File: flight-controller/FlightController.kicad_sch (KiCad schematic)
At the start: 30 parts, among them J1 USB_C_Receptacle_USB2.0_14P, J2 Conn_01x03_Pin, J3 Conn_01x03_Pin, J4 Conn_01x03_Pin, J5 Conn_01x03_Pin, J7 Micro_SD_Card_Det1, J8 Conn_01x06_Pin, U1 ESP32-S3-WROOM-1, U2 TPS629210DRLR, U3 MMC5983MA, U4 BMI270, U5 BMP581

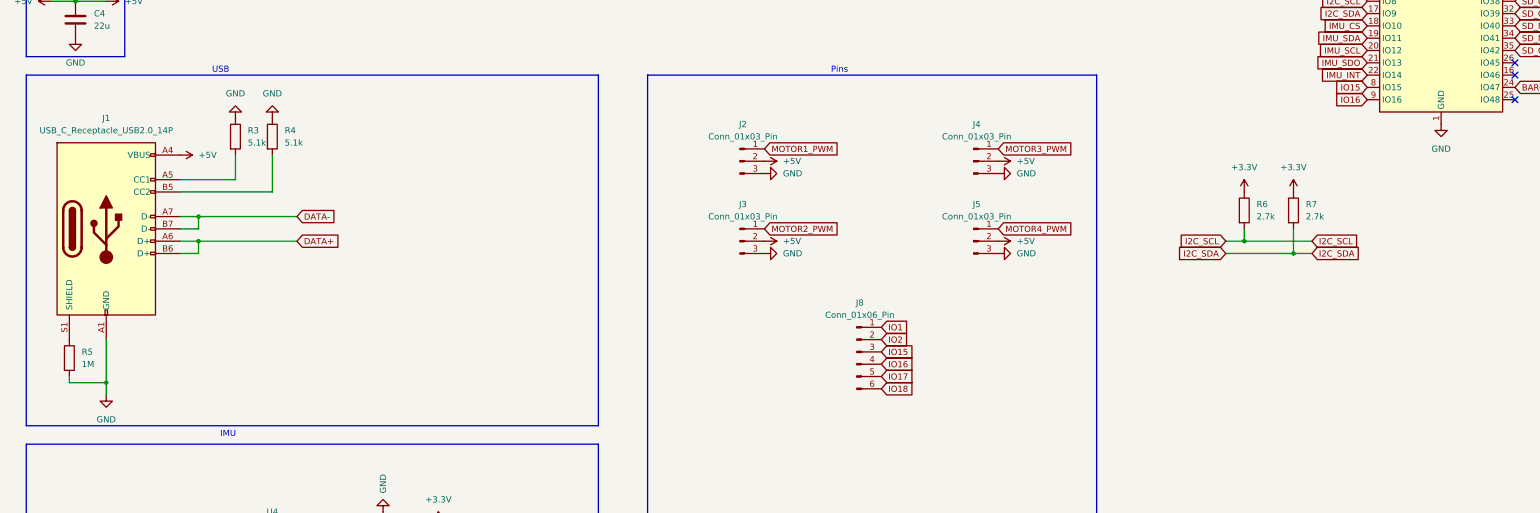
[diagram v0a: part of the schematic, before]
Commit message: update usb
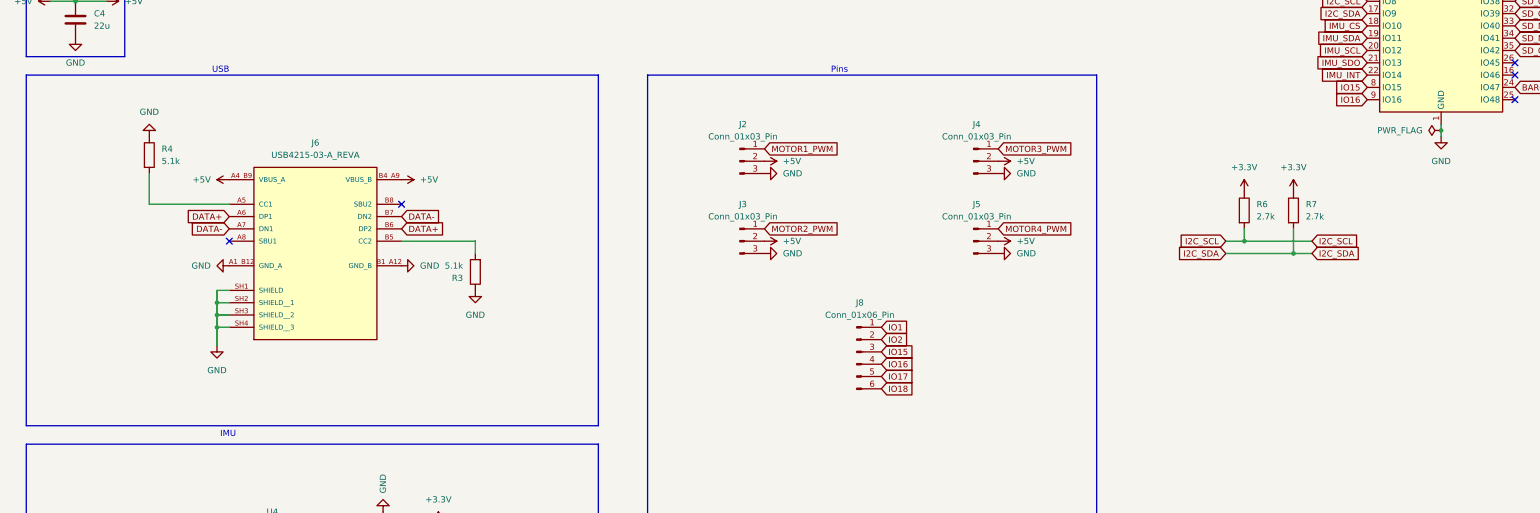
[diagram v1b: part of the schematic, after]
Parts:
- removed J1: USB_C_Receptacle_USB2.0_14P, symbol Connector:USB_C_Receptacle_USB2.0_14P
- removed R5: 1M, symbol Device:R
- added J6: USB4215-03-A_REVA, USB4215-03-A_REVA:GCT_USB4215-03-A_REVA, symbol USB4215-03-A_REVA:USB4215-03-A_REVA
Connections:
- net +5V: now also J6.A4_B9 (VBUS_A), J6.B4_A9 (VBUS_B)
- net DATA+: now also J6.A6 (DP1), J6.B6 (DP2)
- net DATA-: now also J6.A7 (DN1), J6.B7 (DN2)
- net GND: now also J6.A1_B12 (GND_A), J6.B1_A12 (GND_B), J6.SH1 (SHIELD), J6.SH2 (SHIELD__1), J6.SH3 (SHIELD__2), J6.SH4 (SHIELD__3)
- net at R3.2: now also J6.B5 (CC2)
- net at R4.2: now also J6.A5 (CC1)
- no-connect marks 21 -> 23
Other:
- moved on the sheet: R4

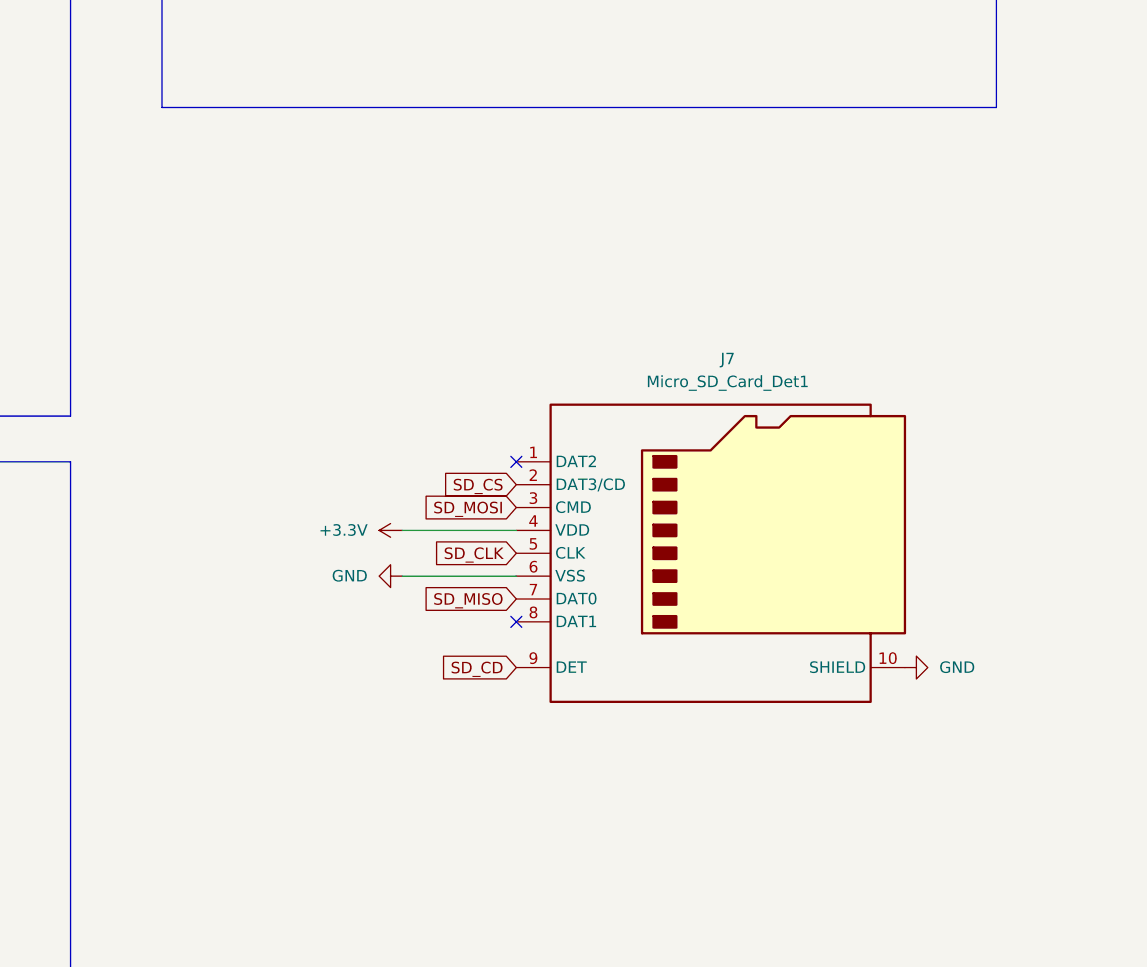
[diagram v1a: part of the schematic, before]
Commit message: add footprints
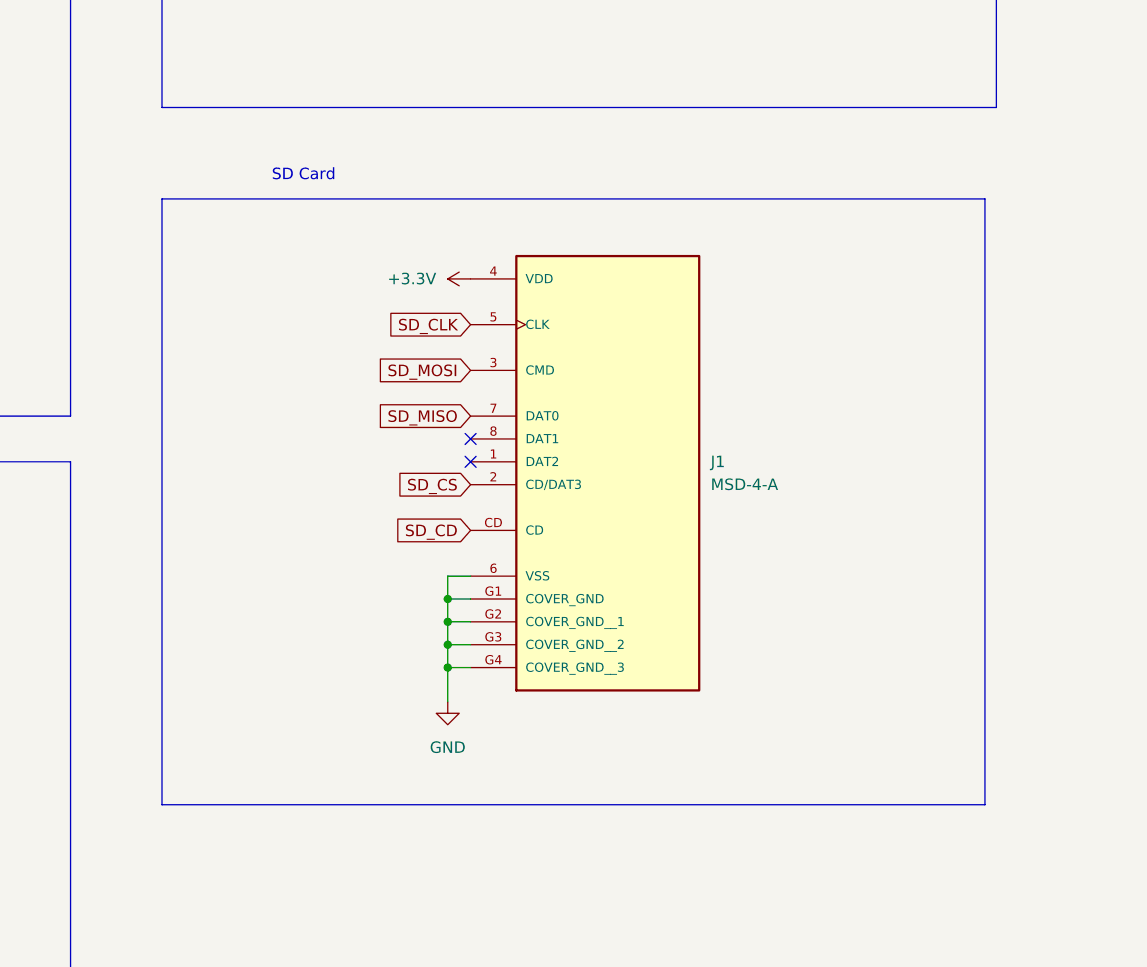
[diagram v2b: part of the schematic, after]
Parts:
- removed J7: Micro_SD_Card_Det1, symbol Connector:Micro_SD_Card_Det1
- added J1: MSD-4-A, MSD-4-A:CUI_MSD-4-A, symbol MSD-4-A:MSD-4-A
- C1, C10, C2, C3, C4, C5, C6, C7, C8, C9: footprint (none) -> Capacitor_SMD:C_0603_1608Metric_Pad1.08x0.95mm_HandSolder
- J2, J3, J4, J5: footprint (none) -> Connector_PinHeader_2.54mm:PinHeader_1x03_P2.54mm_Vertical
- J8: footprint (none) -> Connector_PinHeader_2.54mm:PinHeader_1x06_P2.54mm_Vertical
- L1: footprint (none) -> Inductor_SMD:L_1008_2520Metric_Pad1.43x2.20mm_HandSolder
- R1, R2, R3, R4, R6, R7: footprint (none) -> Resistor_SMD:R_0603_1608Metric_Pad0.98x0.95mm_HandSolder
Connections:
- net +3.3V: now also J1.4 (VDD)
- net GND: now also J1.6 (VSS), J1.G1 (COVER_GND), J1.G2 (COVER_GND__1), J1.G3 (COVER_GND__2), J1.G4 (COVER_GND__3)
- net SD_CD: now also J1.CD
- net SD_CLK: now also J1.5 (CLK)
- net SD_CS: now also J1.2 (CD/DAT3)
- net SD_MISO: now also J1.7 (DAT0)
- net SD_MOSI: now also J1.3 (CMD)
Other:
- note added: "SD Card"

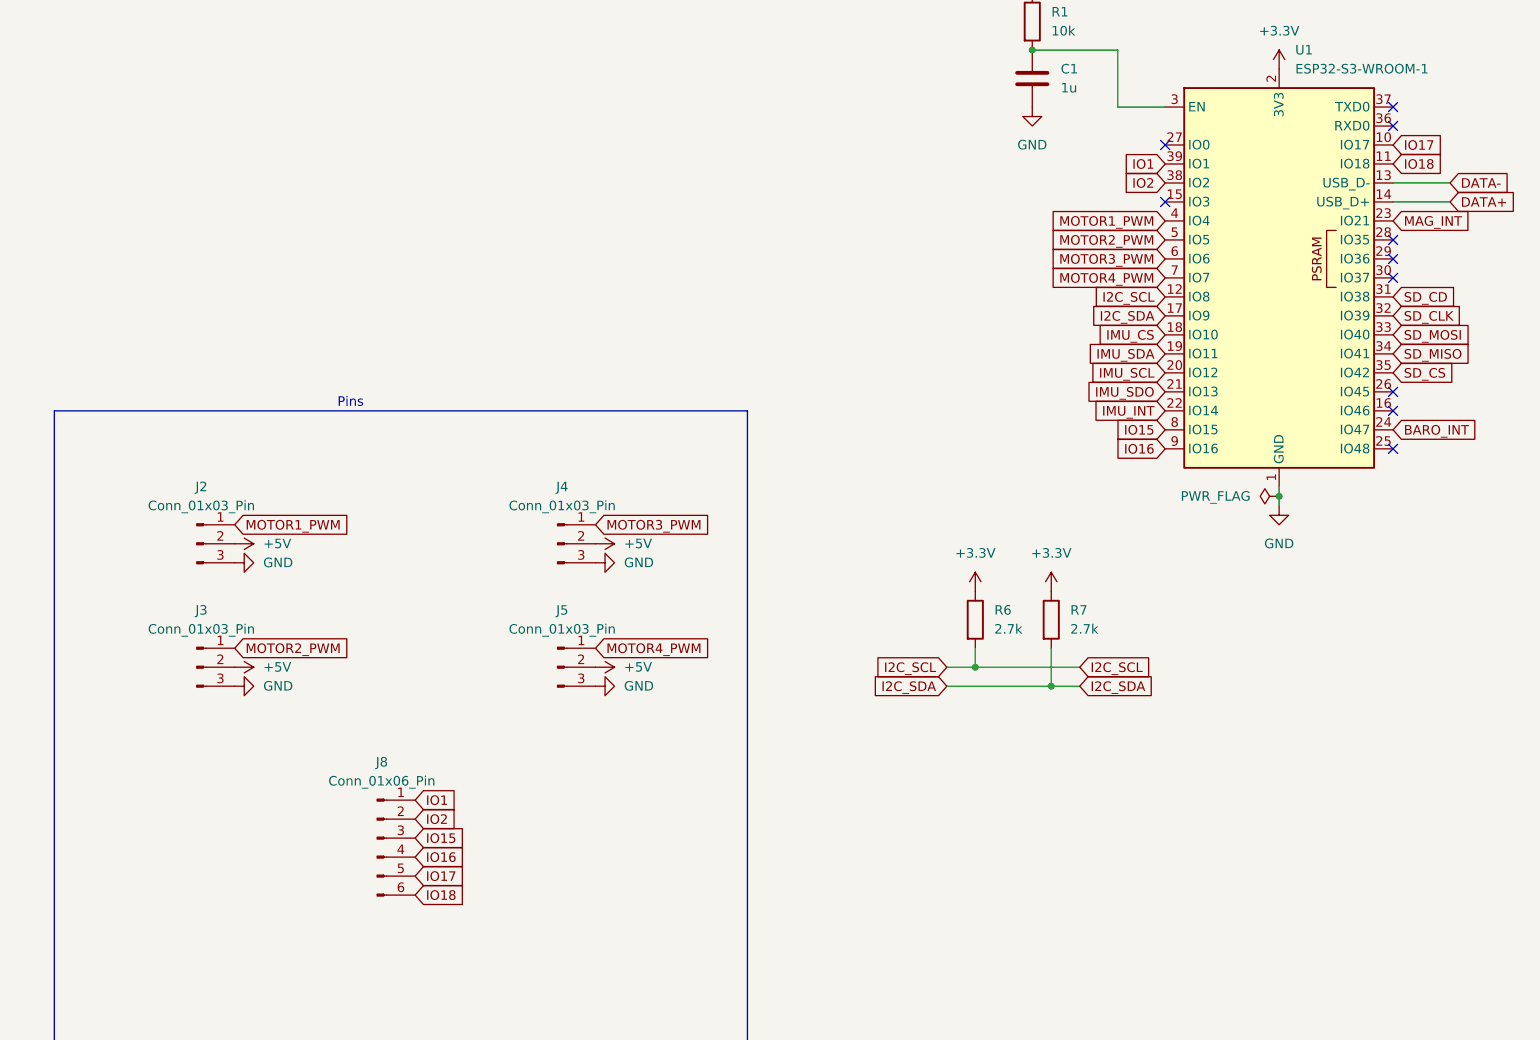
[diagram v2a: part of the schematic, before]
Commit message: general component locations
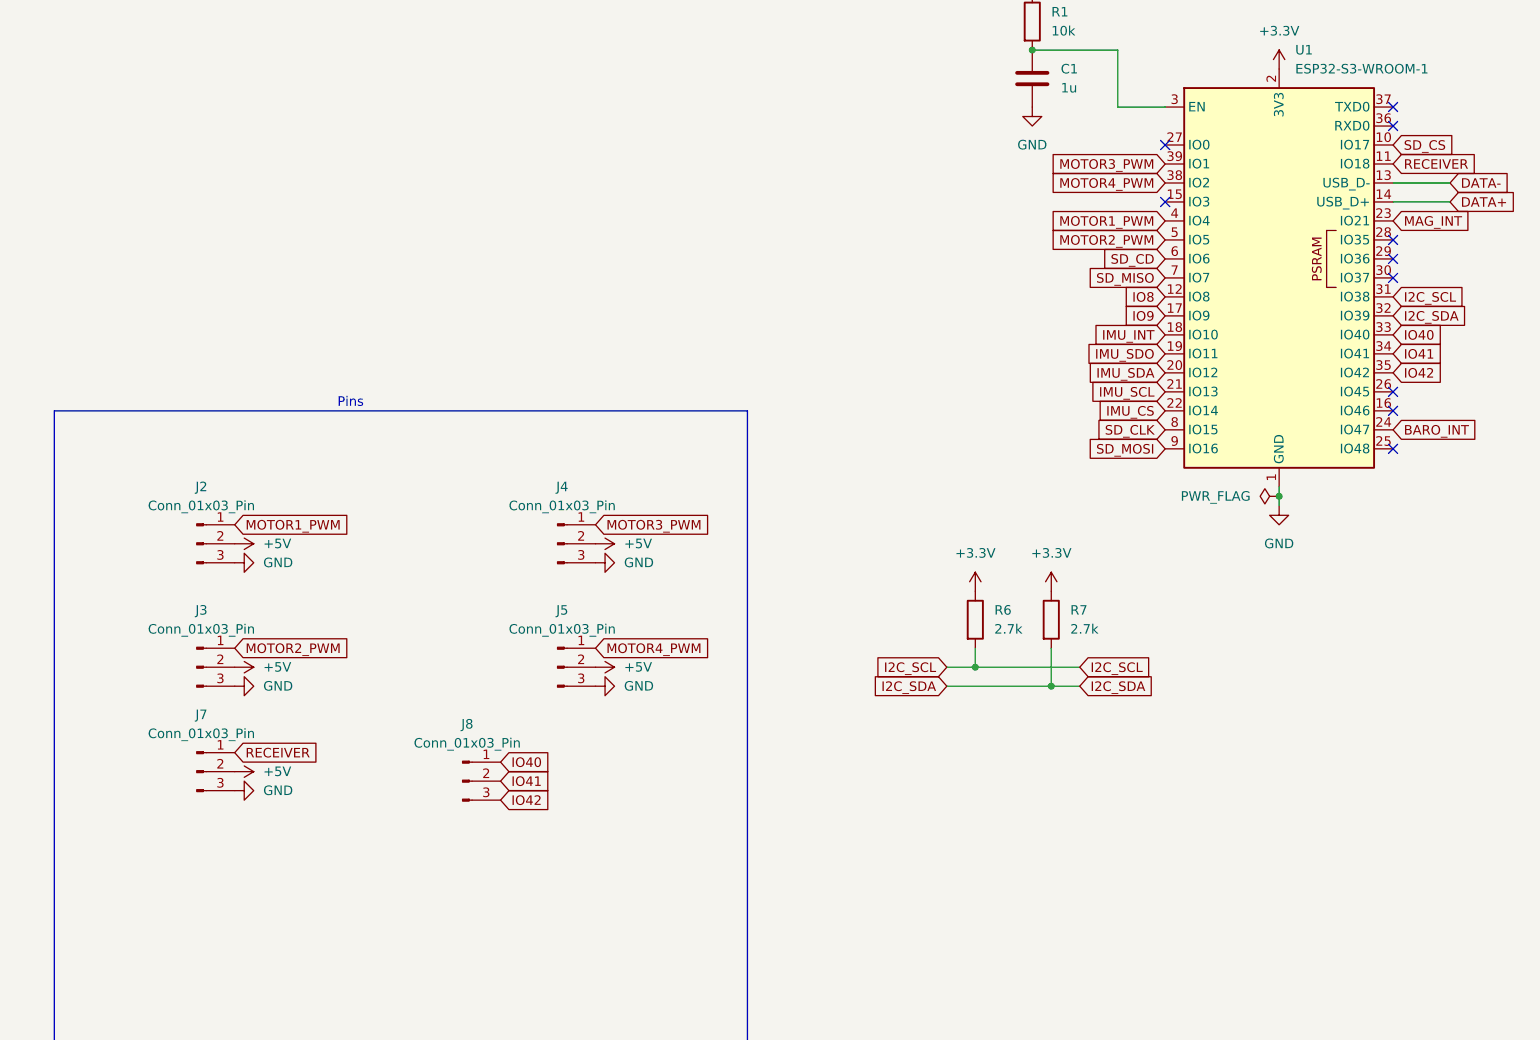
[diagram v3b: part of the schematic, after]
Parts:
- removed J8: Conn_01x06_Pin, Connector_PinHeader_2.54mm:PinHeader_1x06_P2.54mm_Vertical, symbol Connector:Conn_01x06_Pin
- added J7, J8: Conn_01x03_Pin, Connector_PinHeader_2.54mm:PinHeader_1x03_P2.54mm_Vertical, symbol Connector:Conn_01x03_Pin
- J1: footprint MSD-4-A:CUI_MSD-4-A -> MSD_4_A:CUI_MSD-4-A
- J6: footprint USB4215-03-A_REVA:GCT_USB4215-03-A_REVA -> USB4215_03_A:GCT_USB4215-03-A_REVA
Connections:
- net IO1 is gone; now on net MOTOR3_PWM: U1.39 (IO1)
- net IO15 is gone; now on net SD_CLK: U1.8 (IO15)
- net IO16 is gone; now on net SD_MOSI: U1.9 (IO16)
- net IO17 is gone; now on net SD_CS: U1.10 (IO17)
- net IO2 is gone; now on net MOTOR4_PWM: U1.38 (IO2)
- net +5V: now also J7.2 (Pin_2)
- net GND: now also J7.3 (Pin_3)
- net I2C_SCL: now also U1.31 (IO38); no longer U1.12 (IO8)
- net I2C_SDA: now also U1.32 (IO39); no longer U1.17 (IO9)
- net IMU_CS: now also U1.22 (IO14); no longer U1.18 (IO10)
- net IMU_INT: now also U1.18 (IO10); no longer U1.22 (IO14)
- net IMU_SCL: now also U1.21 (IO13); no longer U1.20 (IO12)
- net IMU_SDA: now also U1.20 (IO12); no longer U1.19 (IO11)
- net IMU_SDO: now also U1.19 (IO11); no longer U1.21 (IO13)
- net MOTOR3_PWM: no longer U1.6 (IO6)
- net MOTOR4_PWM: no longer U1.7 (IO7)
- net SD_CD: now also U1.6 (IO6); no longer U1.31 (IO38)
- net SD_CLK: no longer U1.32 (IO39)
- net SD_CS: no longer U1.35 (IO42)
- net SD_MISO: now also U1.7 (IO7); no longer U1.34 (IO41)
- net SD_MOSI: no longer U1.33 (IO40)
- net IO18 renamed RECEIVER
- net RECEIVER: now also J7.1 (Pin_1)
- new net IO40: J8.1 (Pin_1), U1.33 (IO40)
- new net IO41: J8.2 (Pin_2), U1.34 (IO41)
- new net IO42: J8.3 (Pin_3), U1.35 (IO42)
- new net IO8: U1.12 (IO8)
- new net IO9: U1.17 (IO9)
